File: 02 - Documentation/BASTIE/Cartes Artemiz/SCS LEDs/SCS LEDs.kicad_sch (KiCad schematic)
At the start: 16 parts, among them J1 2P Droit 2-11-2022, J2 2P Droit 2-11-2022, K1 SSR CPC1394GR, U1 ${SIM.PARAMS}, U2 Opamp_Dual, U3 Alim LP TSR_0.5-2450

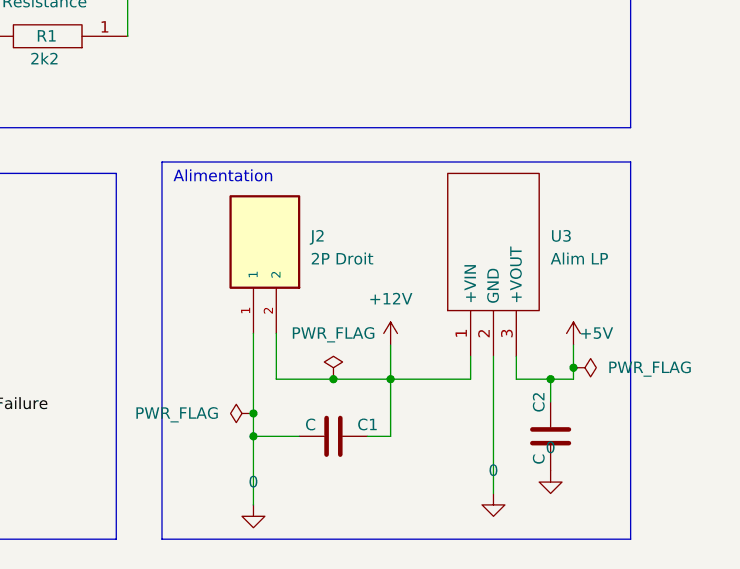
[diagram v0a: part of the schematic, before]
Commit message: Encore qlq corrections
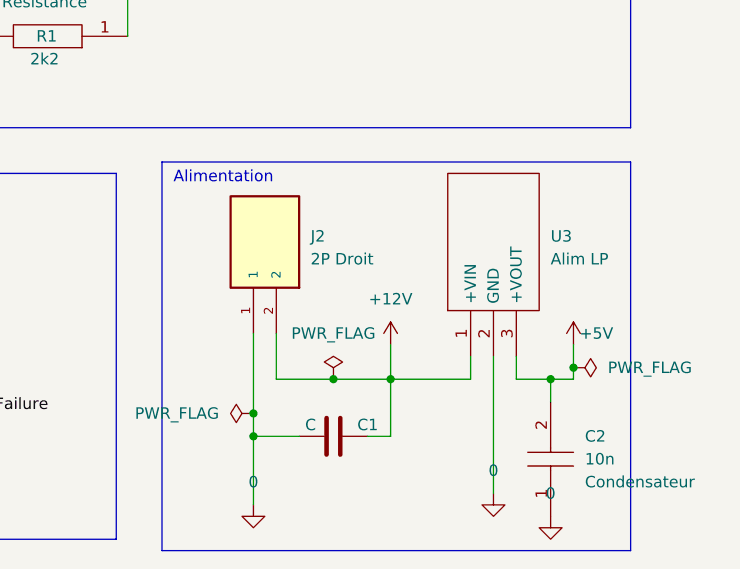
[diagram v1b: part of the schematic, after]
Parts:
- removed C2: C, Capacitor_THT:CP_Radial_D5.0mm_P2.00mm, symbol Device:C
- added C2: 10n, EPSA_lib:CAPC2012X130N, symbol EPSA_lib:Condensateur 0805Y1000104JXT
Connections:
- net +5V: now also C2.2
- net GND: now also C2.1
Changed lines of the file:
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@@
     (stroke (width 0) (type default))
   )
-  (polyline (pts (xy 173.99 151.13) (xy 226.06 151.13))
+  (polyline (pts (xy 173.99 152.4) (xy 226.06 152.4))
     (stroke (width 0) (type default))
   )
@@
     (stroke (width 0) (type default))
   )
-  (polyline (pts (xy 173.99 109.22) (xy 173.99 151.13))
+  (polyline (pts (xy 173.99 109.22) (xy 173.99 152.4))
     (stroke (width 0) (type default))
   )
@@
     (stroke (width 0) (type default))
   )
-  (polyline (pts (xy 226.06 151.13) (xy 226.06 109.22))
+  (polyline (pts (xy 226.06 152.4) (xy 226.06 109.22))
     (stroke (width 0) (type default))
   )
@@
     )
   )
+  (symbol (lib_id "EPSA_lib:Condensateur 0805Y1000104JXT") (at 217.17 148.59 90) (unit 1)
+    (in_bom yes) (on_board yes) (dnp no) (fields_autoplaced)
+    (property "Reference" "C2" (at 220.98 139.7 90)
+      (effects (font (size 1.27 1.27)) (justify right))
+    )
+    (property "Value" "10n" (at 220.98 142.24 90)
+      (effects (font (size 1.27 1.27)) (justify right))
+    )
+    (property "Footprint" "EPSA_lib:CAPC2012X130N" (at 217.17 128.27 0)
+      (effects (font (size 1.27 1.27)) (justify left) hide)
+    )
+    (property "Datasheet" "http://docs-europe.electrocomponents.com/webdocs/119d/0900766b8119d7bc.pdf" (at 219.71 128.27 0)
+      (effects (font (size 1.27 1.27)) (justify left) hide)
+    )
+    (property "Sim.Pins" "1=+ 2=-" (at 214.884 123.444 0)
+      (effects (font (size 1.27 1.27)) hide)
+    )
+    (property "Sim.Device" "C" (at 212.09 128.27 0)
+      (effects (font (size 1.27 1.27)) (justify left) hide)
+    )
+    (property "Description" "Syfer 0805 Ceramic Chip Capacitors" (at 222.25 128.27 0)
+      (effects (font (size 1.27 1.27)) (justify left) hide)
+    )
+    (property "Height" "1.3" (at 224.79 128.27 0)
+      (effects (font (size 1.27 1.27)) (justify left) hide)
+    )
+    (property "Manufacturer_Name" "Syfer" (at 227.33 128.27 0)
+      (effects (font (size 1.27 1.27)) (justify left) hide)
+    )
+    (property "Manufacturer_Part_Number" "0805Y1000104JXT" (at 229.87 128.27 0)
+      (effects (font (size 1.27 1.27)) (justify left) hide)
+    )
+    (property "Mouser Part Number" "" (at 231.14 139.7 0)
+      (effects (font (size 1.27 1.27)) (justify left) hide)
+    )
+    (property "Mouser Price/Stock" "" (at 229.87 128.27 0)
+      (effects (font (size 1.27 1.27)) (justify left) hide)
+    )
+    (property "Render Name" "Condensateur" (at 220.98 144.78 90)
+      (effects (font (size 1.27 1.27)) (justify right))
+    )
+    (pin "1")
+    (pin "2")
+    (instances
+      (project "SCS LEDs"
+        (path "/517051b6-4db9-459f-9eb8-ac2447aa7de0"
+          (reference "C2") (unit 1)
+        )
+      )
+    )
+  )
   (symbol (lib_id "power:+12V") (at 172.72 83.82 90) (unit 1)
     (in_bom yes) (on_board yes) (dnp no) (fields_autoplaced)
@@
     )
   )
-  (symbol (lib_id "power:GND") (at 217.17 143.51 0) (unit 1)
-    (in_bom yes) (on_board yes) (dnp no) (fields_autoplaced)
-    (property "Reference" "#GND06" (at 217.17 146.05 0)
-      (effects (font (size 1.27 1.27)) hide)
-    )
-    (property "Value" "0" (at 217.17 140.97 0)
-      (effects (font (size 1.27 1.27)))
-    )
-    (property "Footprint" "" (at 217.17 143.51 0)
-      (effects (font (size 1.27 1.27)) hide)
-    )
-    (property "Datasheet" "~" (at 217.17 143.51 0)
+  (symbol (lib_id "power:GND") (at 217.17 148.59 0) (unit 1)
+    (in_bom yes) (on_board yes) (dnp no) (fields_autoplaced)
+    (property "Reference" "#GND06" (at 217.17 151.13 0)
+      (effects (font (size 1.27 1.27)) hide)
+    )
+    (property "Value" "0" (at 217.17 146.05 0)
+      (effects (font (size 1.27 1.27)))
+    )
+    (property "Footprint" "" (at 217.17 148.59 0)
+      (effects (font (size 1.27 1.27)) hide)
+    )
+    (property "Datasheet" "~" (at 217.17 148.59 0)
       (effects (font (size 1.27 1.27)) hide)
     )
@@
         )
       )
-    )
-  )
-  (symbol (lib_id "Device:C") (at 217.17 139.7 180) (unit 1)
-    (in_bom yes) (on_board yes) (dnp no)
-    (property "Reference" "C2" (at 215.9 135.89 90)
-      (effects (font (size 1.27 1.27)))
-    )
-    (property "Value" "C" (at 215.9 142.24 90)
-      (effects (font (size 1.27 1.27)))
-    )
-    (property "Footprint" "Capacitor_THT:CP_Radial_D5.0mm_P2.00mm" (at 216.2048 135.89 0)
-      (effects (font (size 1.27 1.27)) hide)
-    )
-    (property "Datasheet" "~" (at 217.17 139.7 0)
-      (effects (font (size 1.27 1.27)) hide)
-    )
-    (pin "1")
-    (pin "2")
-    (instances
-      (project "SCS LEDs"
-        (path "/517051b6-4db9-459f-9eb8-ac2447aa7de0"
-          (reference "C2") (unit 1)
-        )
-      )
-      (project "AMS_IMD_Reset"
-        (path "/7d9bad3e-6cf2-4a61-8644-78bfbb2e310d"
-          (reference "C3") (unit 1)
-        )
-      )
-      (project "Discharge Controller"
-        (path "/aef688cc-a50d-4496-8d50-e7a8695060e9"
-          (reference "C2") (unit 1)
-        )
-      )
